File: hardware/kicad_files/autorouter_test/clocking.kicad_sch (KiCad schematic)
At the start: 4 parts, among them U11 SI5351A-B-GTR, X2 NX3225GA-25_000M-STD-CRG-2

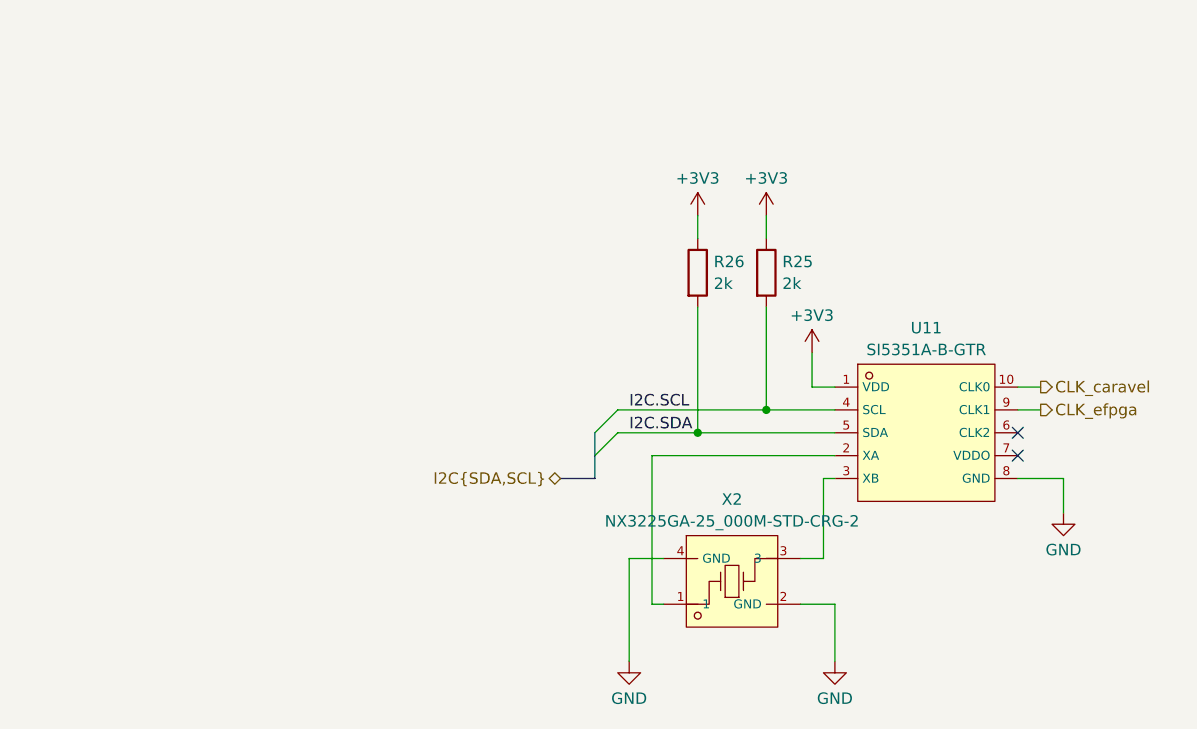
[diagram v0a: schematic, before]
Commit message: feat: first version of a complete layout. USB-C port might be problematic, FTDI chip does not have the best arrangement
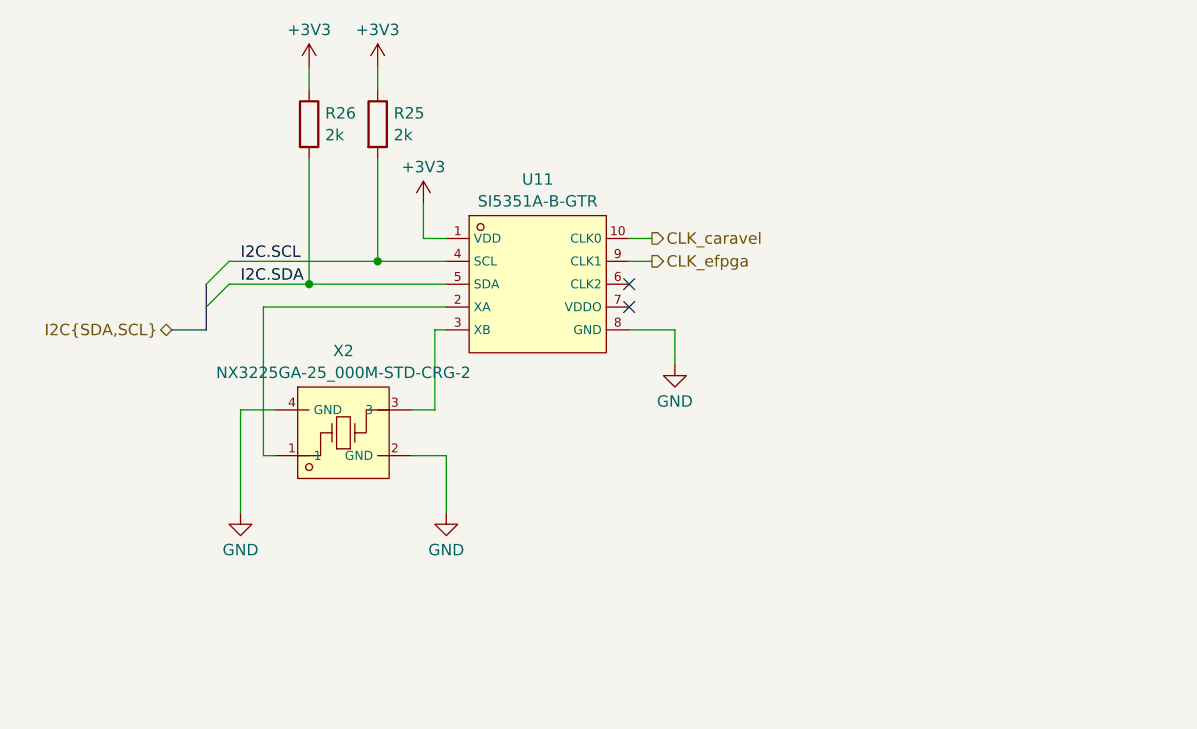
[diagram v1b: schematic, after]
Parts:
- U11: footprint Package_SO:MSOP-10_3x3mm_P0.5mm -> ../../GitHubProjects/FABulous_board/kicad_files/external_libs/easy_eda:MSOP-10_L3.0-W3.0-P0.50-LS5.0-BL
- X2: footprint easy_eda:CRYSTAL-SMD_4P-L3.2-W2.5-BL -> ../../GitHubProjects/FABulous_board/kicad_files/external_libs/easy_eda:CRYSTAL-SMD_4P-L3.2-W2.5-BL
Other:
- title: Clocking -> (none)
- moved on the sheet: R25, R26, U11, X2
